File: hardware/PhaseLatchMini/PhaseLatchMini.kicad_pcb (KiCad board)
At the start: 4 copper layers, 59.7 x 20.3 mm, 47 parts, among them J1 Conn_01x17_Pin, J2 NC, J20 I_IN, J21 Q_IN, J3 Conn_01x17_Pin, J4 USB2.0_16P, J5 Boot, J6 NC, SW3 BTN, U1 STM32F103C8Tx, U5 MIC5504-3.3YM5, Y1 8MHz, Y2 32768Hz

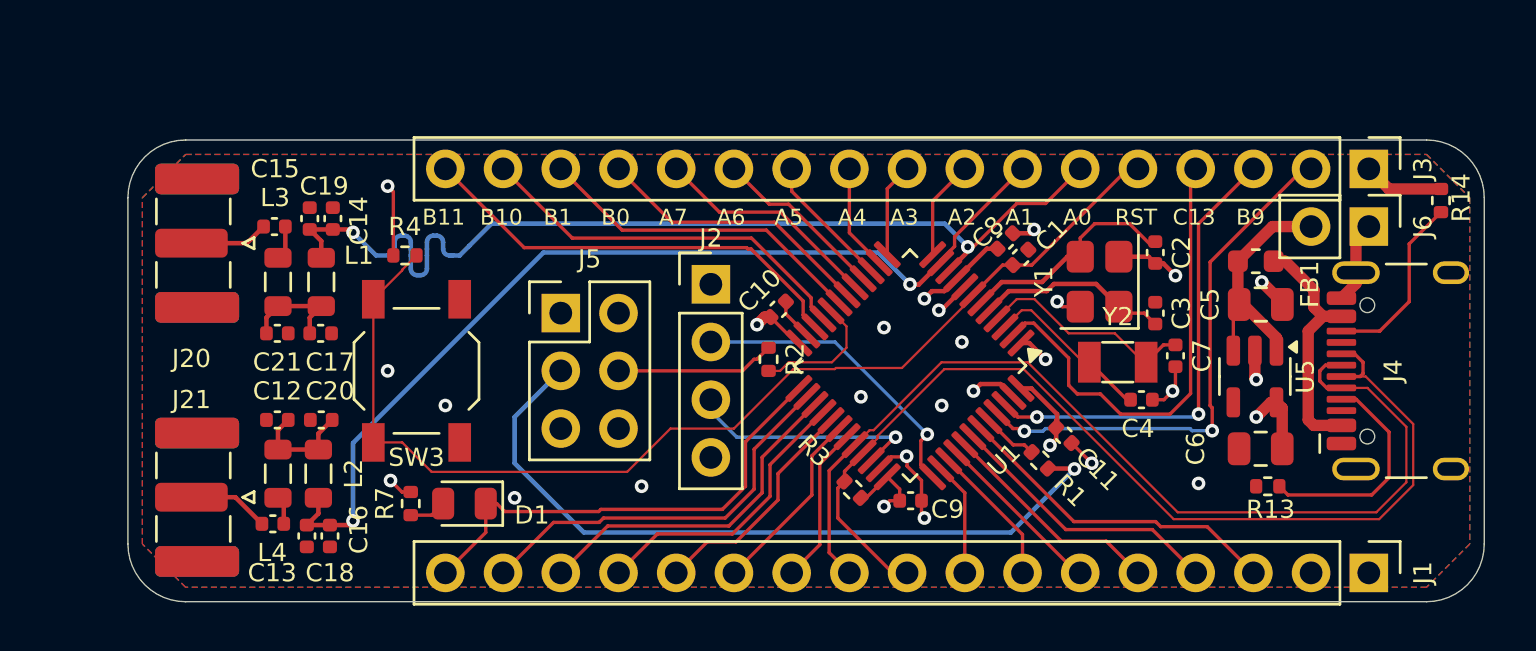
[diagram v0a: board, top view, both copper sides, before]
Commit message: Almost ready for initial release
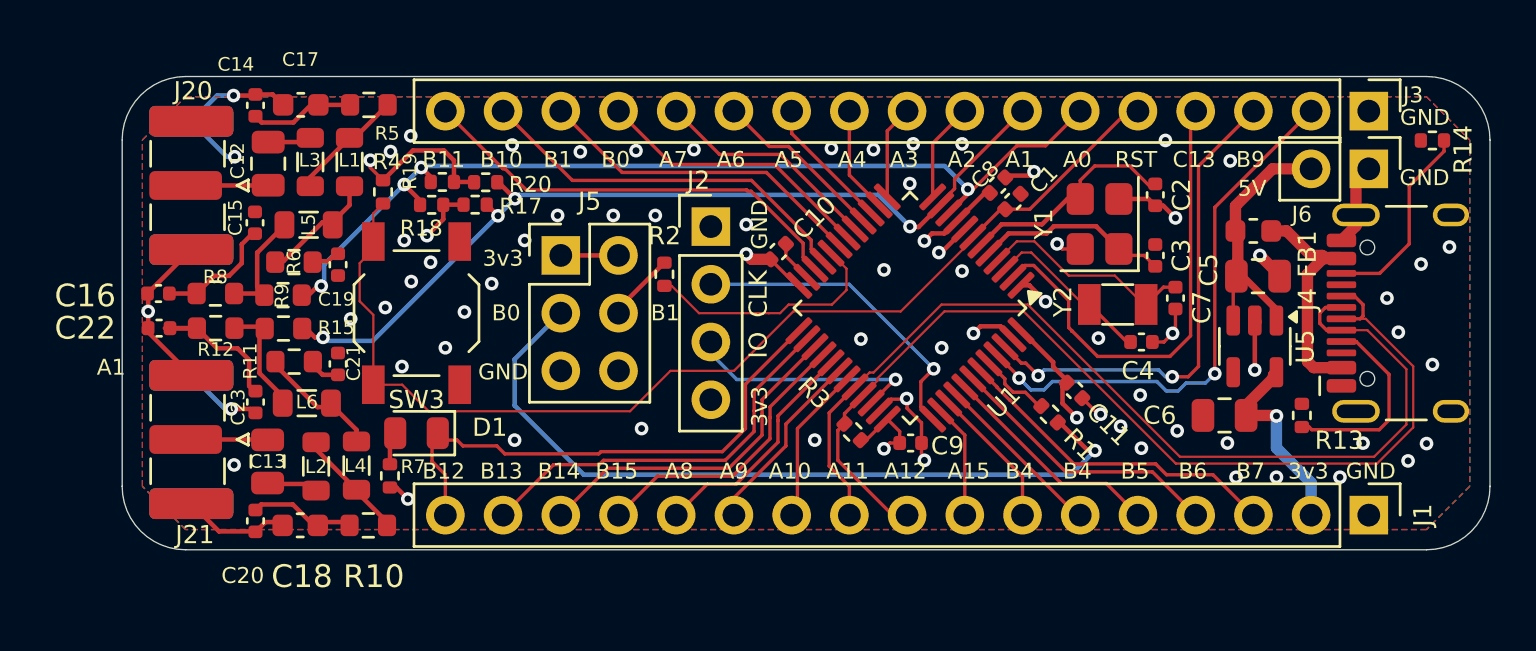
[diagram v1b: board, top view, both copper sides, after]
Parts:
- added C22: 22nF, Capacitor_SMD:C_0402_1005Metric, F.Cu at (150.0, 74.3)
- added C23: 100nF, Capacitor_SMD:C_0402_1005Metric, F.Cu at (154.2, 77.6)
- added L5: 10uH, Inductor_SMD:L_0805_2012Metric, F.Cu at (156.5, 69.8)
- added L6: 10uH, Inductor_SMD:L_0805_2012Metric, F.Cu at (156.5, 77.6)
- added R10: 4.7, Resistor_SMD:R_0603_1608Metric, F.Cu at (159.2, 83.0)
- added R11: 4.7, Resistor_SMD:R_0603_1608Metric, F.Cu at (155.9, 75.8)
- added R12: 4.7, Resistor_SMD:R_0603_1608Metric, F.Cu at (152.5, 74.3)
- added R15: 10, Resistor_SMD:R_0603_1608Metric, F.Cu at (155.4, 74.3)
- added R17: NC, Resistor_SMD:R_0402_1005Metric, F.Cu at (163.9, 68.9)
- added R18: NC, Resistor_SMD:R_0402_1005Metric, F.Cu at (162.0, 68.9)
- added R19: NC, Resistor_SMD:R_0402_1005Metric, F.Cu at (162.4, 67.9)
- added R20: NC, Resistor_SMD:R_0402_1005Metric, F.Cu at (164.3, 67.9)
- added R5: 4.7, Resistor_SMD:R_0603_1608Metric, F.Cu at (159.2, 64.5)
- added R6: 4.7, Resistor_SMD:R_0603_1608Metric, F.Cu at (155.9, 71.4)
- added R8: 4.7, Resistor_SMD:R_0603_1608Metric, F.Cu at (152.4, 72.8)
- added R9: 10, Resistor_SMD:R_0603_1608Metric, F.Cu at (155.4, 72.9)
- C12: value 22nF -> 1uF; footprint Capacitor_SMD:C_0402_1005Metric -> Capacitor_SMD:C_0805_2012Metric
- C13: value 100nF -> 1uF; footprint Capacitor_SMD:C_0402_1005Metric -> Capacitor_SMD:C_0805_2012Metric
- C15: value 100nF -> 22nF
- C16: value 22nF -> 100nF
- C17, C18: value 22nF -> 470nF; footprint Capacitor_SMD:C_0402_1005Metric -> Capacitor_SMD:C_0603_1608Metric
- C19, C21: value 22nF -> 220nF
- moved C16 13.1 mm to (149.9, 72.8), turned to 180 degrees
- moved C12 11.3 mm to (154.8, 67.1), turned to 90 degrees
- moved C17 10.1 mm to (156.2, 64.5), turned to 180 degrees
- moved C14 6.03 mm to (154.2, 64.5)
- moved R2 5.92 mm to (172.2, 72.0)
- moved L3 5.47 mm to (156.6, 67.0)
- moved L1 5.42 mm to (158.3, 67.0), turned to -90 degrees
- moved C20 5.30 mm to (154.2, 82.8), turned to -90 degrees
- moved D1 3.75 mm to (161.3, 78.9)
- moved L4 3.47 mm to (158.6, 80.4)
- moved R13 3.46 mm to (200.3, 78.2), turned to 90 degrees
- moved C21 2.99 mm to (157.8, 75.9), turned to 90 degrees
- moved R4 2.96 mm to (159.8, 68.3), turned to 90 degrees
- moved C13 2.75 mm to (154.7, 80.2), turned to -90 degrees
- moved R14 2.67 mm to (206.0, 66.1), turned to 180 degrees
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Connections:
- C12 pad 1: Net-(C12-Pad1) -> Net-(J20-In)
- C12 pad 2: GND -> Net-(C12-Pad2)
- C13 pad 1: Net-(C13-Pad1) -> Net-(J21-In)
- C13 pad 2: Net-(J21-In) -> Net-(C13-Pad2)
- C14 pad 1: /PA0 -> Net-(C14-Pad1)
- C15 pad 2: Net-(J20-In) -> GND
- C16 pad 1: /PA1 -> Net-(C15-Pad1)
- C17 pad 1: Net-(C17-Pad1) -> Net-(C14-Pad1)
- C18 pad 1: /PA1 -> Net-(C18-Pad1)
- C19 pad 1: /PA0 -> Net-(C19-Pad1)
- C20 pad 1: Net-(C12-Pad1) -> Net-(C18-Pad1)
- C21 pad 1: Net-(C17-Pad1) -> Net-(C21-Pad1)
- L1 pad 1: Net-(C17-Pad1) -> Net-(L1-Pad1)
- L1 pad 2: /PA0 -> Net-(L1-Pad2)
- L2 pad 1: Net-(C12-Pad1) -> Net-(C13-Pad2)
- L2 pad 2: /PA1 -> Net-(L2-Pad2)
- L3 pad 1: Net-(C15-Pad1) -> Net-(C12-Pad2)
- L3 pad 2: Net-(C17-Pad1) -> Net-(L1-Pad1)
- L4 pad 1: Net-(C13-Pad1) -> Net-(L2-Pad2)
- L4 pad 2: Net-(C12-Pad1) -> Net-(L4-Pad2)
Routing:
- net GND: track 28.2 -> 50.0 mm, vias 20 -> 68
- net +3V3: track 22.7 -> 34.9 mm
- net Net-(C22-Pad1): track 0.00 -> 6.99 mm
- net Net-(L1-Pad2): track 0.00 -> 5.34 mm
- net Net-(L4-Pad2): track 0.00 -> 5.19 mm
- net Net-(L5-Pad2): track 0.00 -> 5.10 mm
- net /PB2: track 5.76 -> 10.8 mm
- net Net-(L1-Pad1): track 0.00 -> 4.89 mm
- net Net-(C12-Pad1): track 4.82 -> 0.00 mm
- net Net-(C17-Pad1): track 4.72 -> 0.00 mm
- net Net-(L6-Pad2): track 0.00 -> 4.64 mm
- net Net-(L2-Pad2): track 0.00 -> 4.56 mm
- net Net-(C18-Pad1): track 0.00 -> 4.36 mm
- net Net-(C14-Pad1): track 0.00 -> 4.28 mm
- net /BOOT1: track 7.03 -> 2.86 mm
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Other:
- board size 59.7 x 20.3 mm -> 60.2 x 20.8 mm
- board text added: "3v3"
- board text added: "5V"
- board text added: "A10"
- board text added: "A11"
- board text added: "A12"
- board text added: "A15"
- board text added: "A8"
- board text added: "A9"
- board text added: "B12"
- board text added: "B13"
- board text added: "B14"
- board text added: "B15"
- board text added: "B4"
- board text added: "B5"
- board text added: "B6"
- board text added: "B7"
- board text added: "CLK"
- board text added: "GND"
- board text added: "IO"
- board text added: "Thank you for buying or making this prototype PhaseLatch Mini ABNielsen.com/PhaseLoom"
